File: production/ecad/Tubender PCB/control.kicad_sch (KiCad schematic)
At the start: 2 parts, among them U2 ESP32-WROOM-32UE_M113EH6400UH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, U7 MCP23017_GPIO_EXPANDER

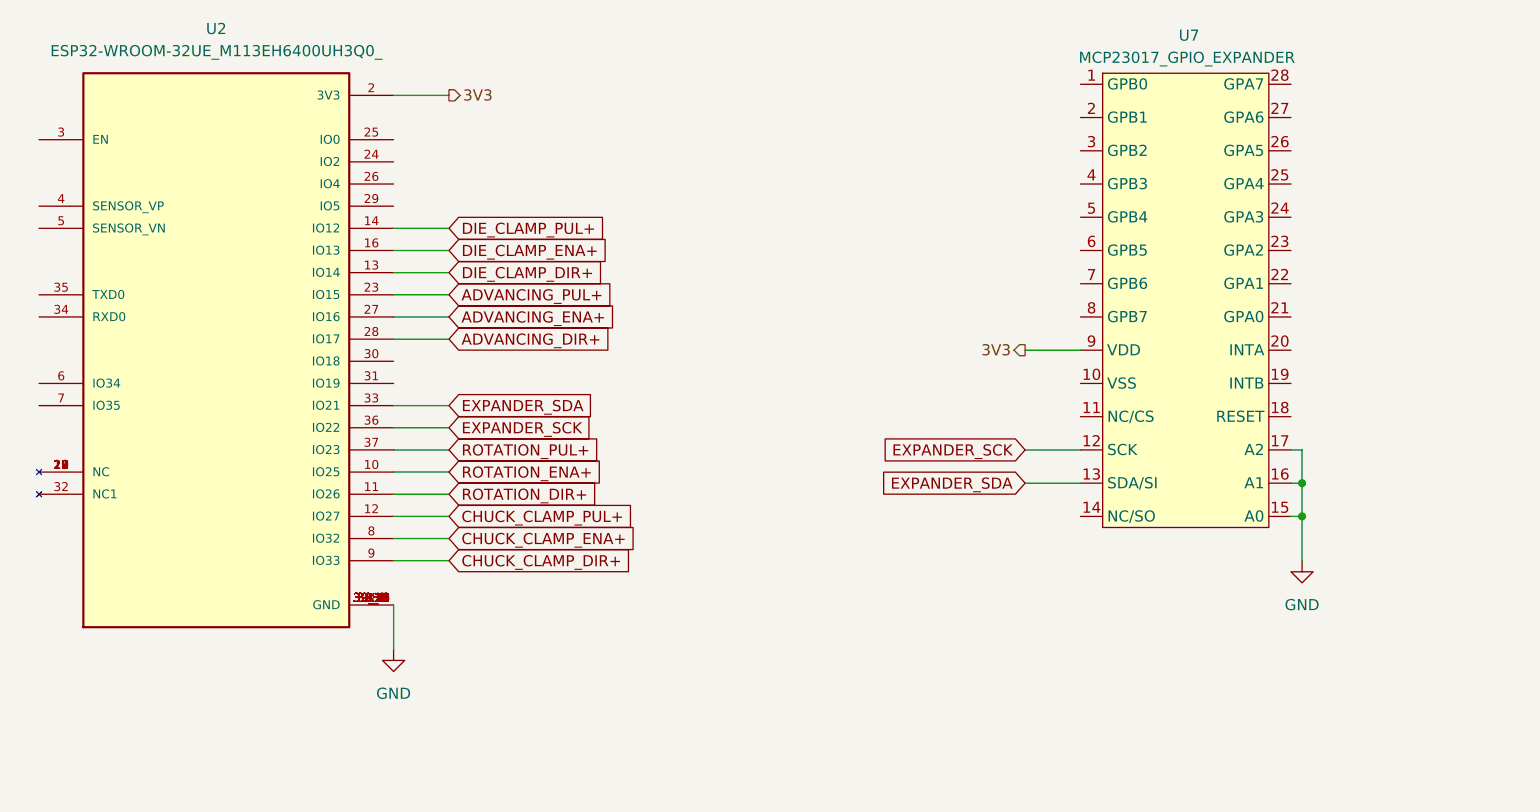
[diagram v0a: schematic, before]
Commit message: MCU and such
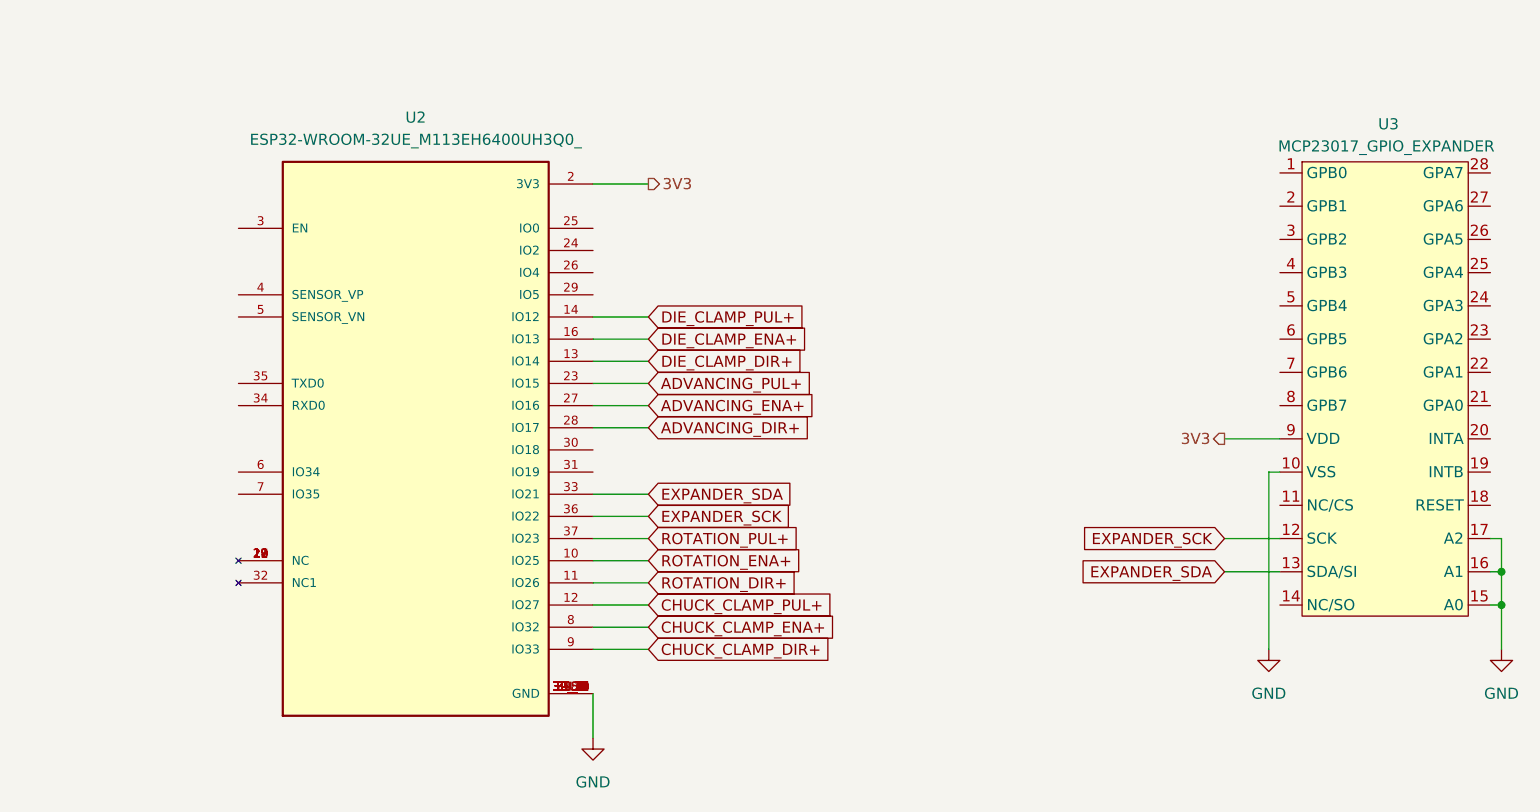
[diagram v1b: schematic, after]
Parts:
- removed U7: MCP23017_GPIO_EXPANDER, symbol MCP23017:MCP23017_GPIO_EXPANDER
- added U3: MCP23017_GPIO_EXPANDER, symbol MCP23017:MCP23017_GPIO_EXPANDER
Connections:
- net 3V3: now also U3.9 (VDD)
- net EXPANDER_SCK: now also U3.12 (SCK)
- net EXPANDER_SDA: now also U3.13 (SDA/SI)
- net GND: now also U3.10 (VSS), U3.15 (A0), U3.16 (A1), U3.17 (A2)

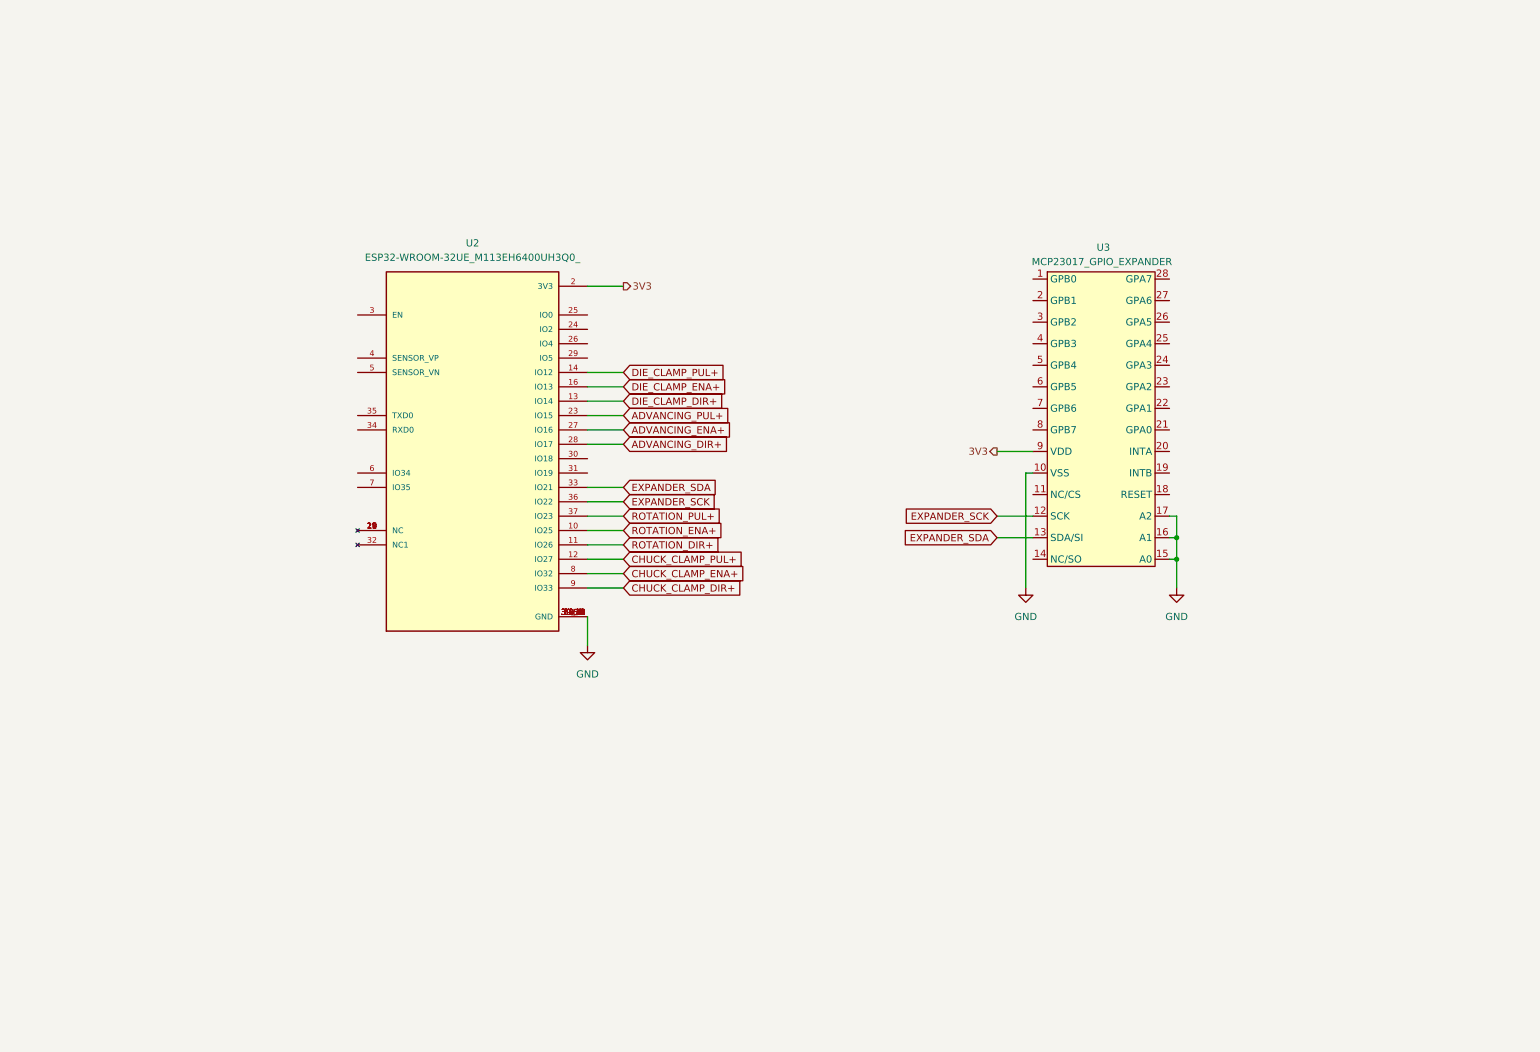
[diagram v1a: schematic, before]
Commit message: More MCU Stuff
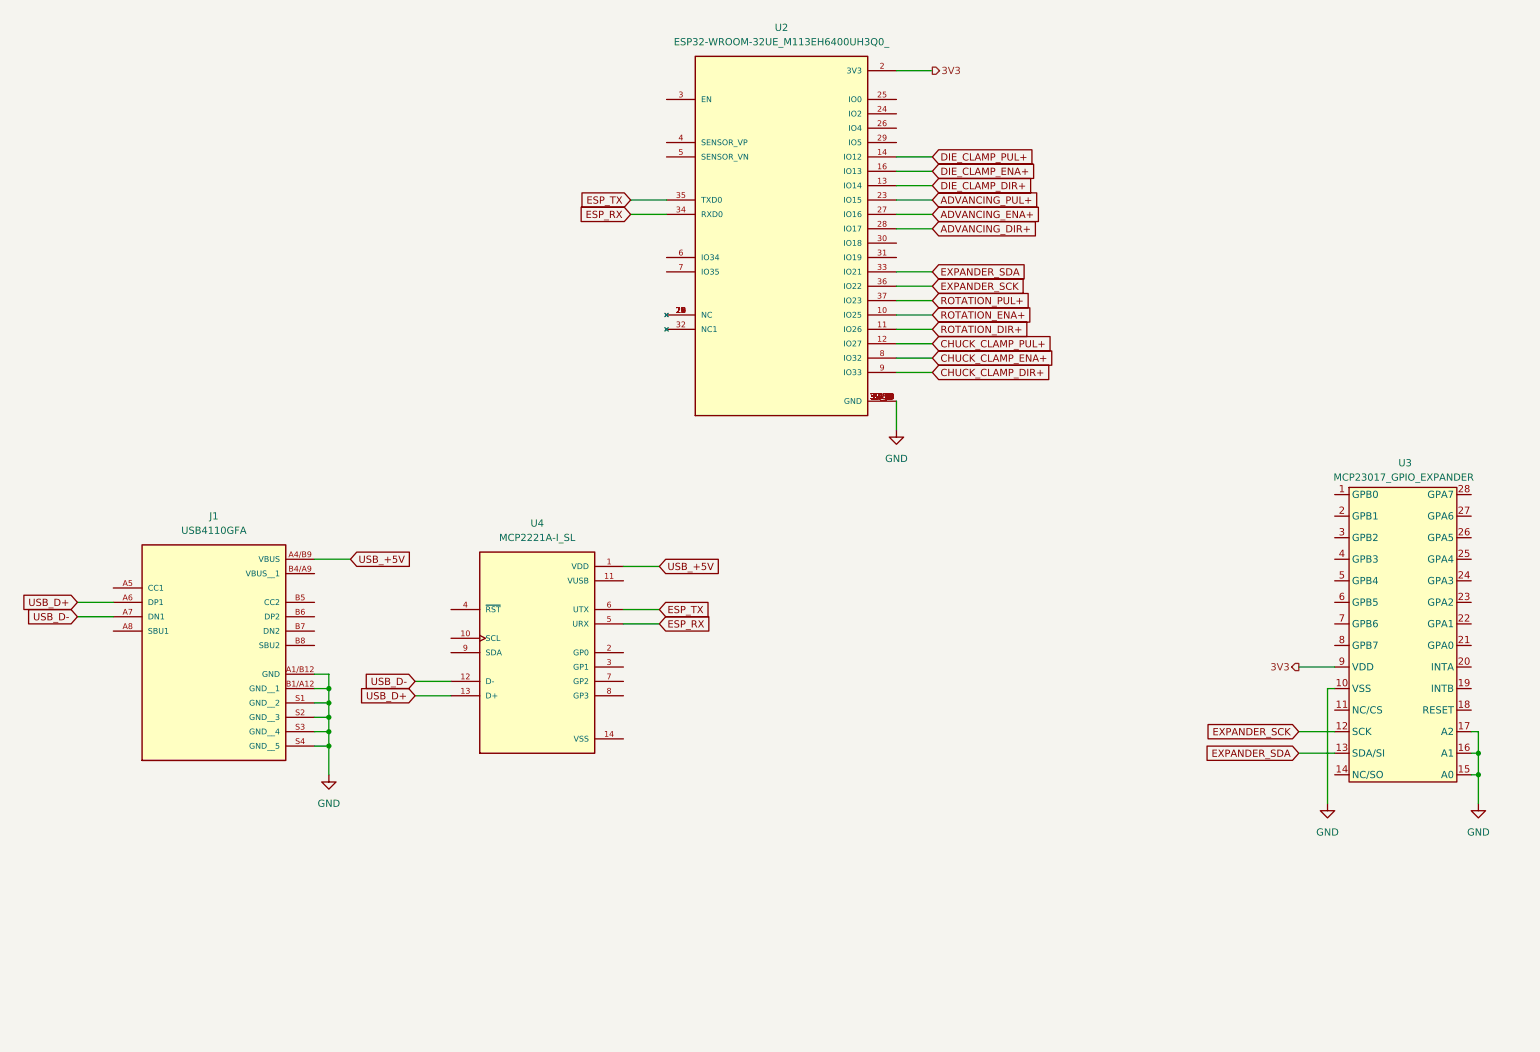
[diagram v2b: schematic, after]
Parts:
- added J1: USB4110GFA, USB4110GFA:GCT_USB4110GFA, symbol USB4110GFA:USB4110GFA
- added U4: MCP2221A-I_SL, MCP2221A-I_SL:SOIC127P600X175-14N, symbol MCP2221A-I_SL:MCP2221A-I_SL
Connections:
- net GND: now also J1.A1/B12 (GND), J1.B1/A12 (GND__1), J1.S1 (GND__2), J1.S2 (GND__3), J1.S3 (GND__4), J1.S4 (GND__5)
- net ESP_RX: now reaches U2.34 (RXD0)
- net ESP_RX: now also U4.5 (URX)
- net ESP_TX: now reaches U2.35 (TXD0)
- net ESP_TX: now also U4.6 (UTX)
- new net USB_+5V: J1.A4/B9 (VBUS), U4.1 (VDD)
- new net USB_D+: J1.A6 (DP1), U4.13 (D+)
- new net USB_D-: J1.A7 (DN1), U4.12 (D-)
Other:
- moved on the sheet: U2, U3

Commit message: MCU Rev1 Complete
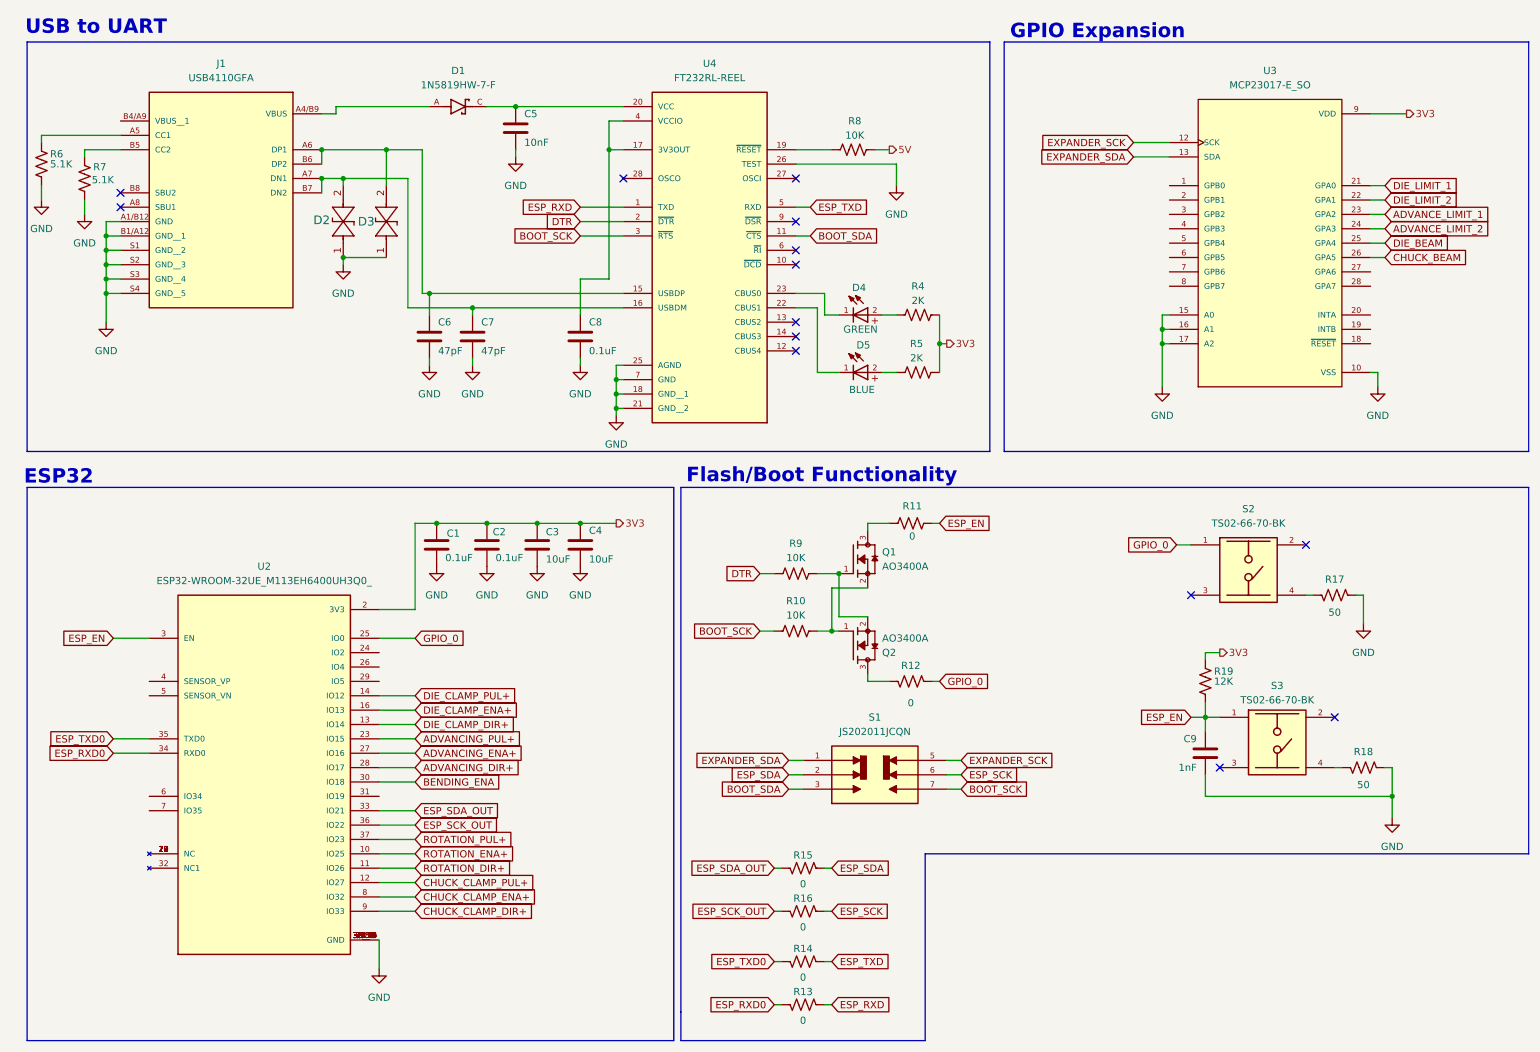
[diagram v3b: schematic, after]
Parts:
- removed U3: MCP23017_GPIO_EXPANDER, symbol MCP23017:MCP23017_GPIO_EXPANDER
- removed U4: MCP2221A-I_SL, MCP2221A-I_SL:SOIC127P600X175-14N, symbol MCP2221A-I_SL:MCP2221A-I_SL
- added C1, C2, C8: 0.1uF, symbol Device:C
- added C3, C4: 10uF, symbol Device:C
- added C5: 10nF, symbol Device:C
- added C6, C7: 47pF, symbol Device:C
- added C9: 1nF, symbol Device:C
- added D1: 1N5819HW-7-F, 1N5819HW-7-F:SOD3715X145N, symbol 1N5819HW-7-F:1N5819HW-7-F
- added D2, D3: RCLAMP1521P.TCT, TVS_DFN2_SLP1006P2_SEM, symbol RCLAMP1521P:RCLAMP1521P.TCT
- added D4: GREEN, WL-SMCW_0603:WL-SMCW_0603, symbol WL-SMCW_0603:WL-SMCW_0603
- added D5: BLUE, WL-SMCW_0603:WL-SMCW_0603, symbol WL-SMCW_0603:WL-SMCW_0603
- added Q1, Q2: AO3400A, AO3400A:SOT95P280X125-3N, symbol AO3400A:AO3400A
- added R10, R8, R9: 10K, symbol Device:R_US
- added R11, R12, R13, R14, R15, R16: 0, symbol Device:R_US
- added R17, R18: 50, symbol Device:R_US
- added R19: 12K, symbol Device:R_US
- added R4, R5: 2K, symbol Device:R_US
- added R6, R7: 5.1K, symbol Device:R_US
- added S1: JS202011JCQN, JS202011JCQN:SW_JS202011JCQN, symbol JS202011JCQN:JS202011JCQN
- added S2, S3: TS02-66-70-BK, TS02-66-70-BK-260-LCR-D:SW_TS02-66-70-BK-260-LCR-D, symbol TS02-66-70-BK-260-LCR-D:TS02-66-70-BK-260-LCR-D
- added U3: MCP23017-E_SO, MCP23017-E_SO:SOIC127P1030X265-28N, symbol MCP23017-E_SO:MCP23017-E_SO
- added U4: FT232RL-REEL, FT232RL-REEL:SOP65P780X200-28N, symbol FT232RL-REEL:FT232RL-REEL
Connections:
- net USB_D+ is gone; now on an unnamed net: J1.A6 (DP1)
- net USB_D- is gone; now on an unnamed net: J1.A7 (DN1)
- net 3V3: now also C1.1, C2.1, C3.1, C4.1, R19.2, R4.2, R5.2, U3.9 (VDD)
- net EXPANDER_SCK: now also S1.5, U3.12 (SCK); no longer U2.36 (IO22)
- net EXPANDER_SDA: now also S1.1, U3.13 (SDA); no longer U2.33 (IO21)
- net GND: now also C1.2, C2.2, C3.2, C4.2, C5.2, C6.2, C7.2, C8.2, C9.2, D2.1, D3.1, R17.2, R18.2, R6.1, R7.1, U3.10 (VSS), U3.15 (A0), U3.16 (A1), U3.17 (A2), U4.18 (GND__1), U4.21 (GND__2), U4.25 (AGND), U4.26 (TEST), U4.7 (GND)
- net GPIO_0: now reaches U2.25 (IO0)
- net GPIO_0: now also R12.2, S2.1
- net ESP_EN: now reaches U2.3 (EN)
- net ESP_EN: now also C9.1, R11.2, R19.1, S3.1
- net BENDING_ENA: now reaches U2.30 (IO18)
- net at J1.A5 (CC1): now also R6.2
- net at J1.B5 (CC2): now also R7.2
- net at J1.B6 (DP2): now also C6.1, D3.2, U4.15 (USBDP)
- net at J1.B7 (DN2): now also C7.1, D2.2, U4.16 (USBDM)
- net ESP_RX renamed ESP_RXD0
- net ESP_RXD0: now also R13.1
- net ESP_TX renamed ESP_TXD0
- net ESP_TXD0: now also R14.1
- net USB_+5V: no longer names the net of J1.A4/B9 (VBUS)
- net USB_+5V: now also D1.A
- new net: Q1.1, Q2.2, R9.2
- new net: Q1.2, Q2.1, R10.2
- new net: Q1.3, R11.1
- new net: R18.1, S3.4
- new net: Q2.3, R12.1
- new net: R8.1, U4.19 (~{RESET})
- new net: C5.1, D1.C, U4.20 (VCC)
- new net: D4.2, R4.1
- new net: R17.1, S2.4
- new net: D4.1, U4.23 (CBUS0)
- new net: C8.1, U4.17 (3V3OUT), U4.4 (VCCIO)
- new net: D5.1, U4.22 (CBUS1)
- new net: D5.2, R5.1
- new net 5V: R8.2
- new net ADVANCE_LIMIT_1: U3.23 (GPA2)
- new net ADVANCE_LIMIT_2: U3.24 (GPA3)
- new net BOOT_SCK: R10.1, S1.7, U4.3 (~{RTS})
- new net BOOT_SDA: S1.3, U4.11 (~{CTS})
- new net CHUCK_BEAM: U3.26 (GPA5)
- new net DIE_BEAM: U3.25 (GPA4)
- new net DIE_LIMIT_1: U3.21 (GPA0)
- new net DIE_LIMIT_2: U3.22 (GPA1)
- new net DTR: R9.1, U4.2 (~{DTR})
- new net ESP_RXD: R13.2, U4.1 (TXD)
- new net ESP_SCK: R16.2, S1.6
- new net ESP_SCK_OUT: R16.1, U2.36 (IO22)
- new net ESP_SDA: R15.2, S1.2
- new net ESP_SDA_OUT: R15.1, U2.33 (IO21)
- new net ESP_TXD: R14.2, U4.5 (RXD)
- no-connect marks 0 -> 14
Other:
- note added: "ESP32"
- note added: "Flash/Boot Functionality"
- note added: "GPIO Expansion"
- note added: "USB to UART"
- moved on the sheet: J1, U2
